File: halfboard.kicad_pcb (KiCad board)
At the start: 2 copper layers, 117.4 x 87.9 mm, 54 parts, among them U1 

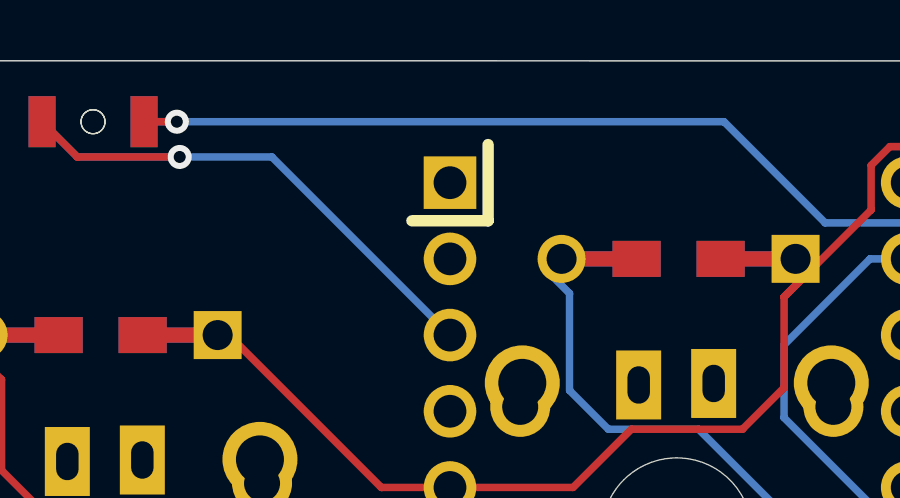
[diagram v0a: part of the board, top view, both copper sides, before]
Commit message: update gerber files
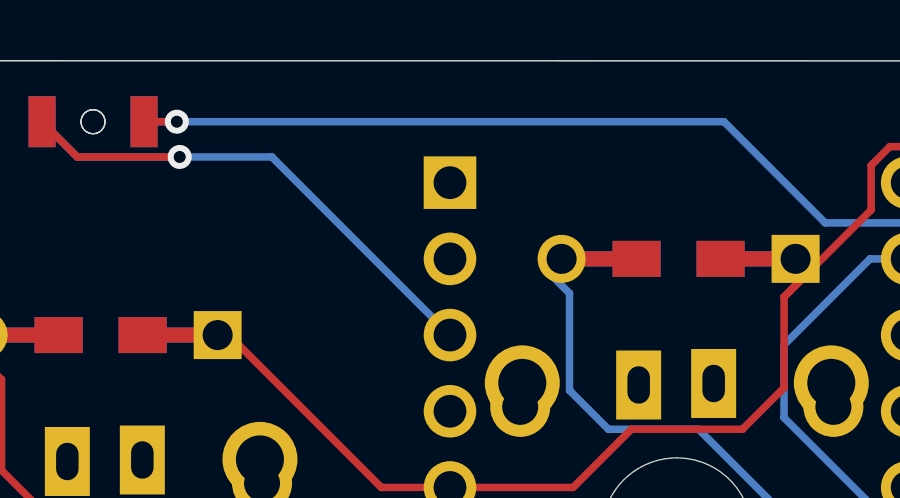
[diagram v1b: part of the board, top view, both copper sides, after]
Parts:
- removed the   at (135.4, 130.6) (x2)
- added  : , Button_Switch_SMD:SW_SPDT_PCM12, F.Cu at (135.4, 130.6)
- added  : , Button_Switch_SMD:SW_SPDT_PCM12, B.Cu at (135.4, 130.6)
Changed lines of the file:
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@@
     (add_net row3)
+  )
+  (module halfboard:ArduinoProMicro-TopSide (layer F.Cu)
+    (at 68.287231 63.5 270)
+    (fp_text reference U1 (at 0 1.625 270) (layer B.SilkS) hide
+      (effects (font (size 1.27 1.524) (thickness 0.2032)) (justify mirror))
+    )
+    (fp_text value " " (at 0 0 270) (layer F.SilkS) hide
+      (effects (font (size 1.27 1.524) (thickness 0.2032)))
+    )
+    (pad 1 thru_hole rect (at -13.97 7.62 270) (size 1.7526 1.7526) (drill 1.0922) (layers *.Cu B.SilkS))
+    (pad 2 thru_hole circle (at -11.43 7.62 270) (size 1.7526 1.7526) (drill 1.0922) (layers *.Cu *.Mask))
+    (pad 3 thru_hole circle (at -8.89 7.62 270) (size 1.7526 1.7526) (drill 1.0922) (layers *.Cu *.Mask)
+      (net 39 RESET_GND))
+    (pad 4 thru_hole circle (at -6.35 7.62 270) (size 1.7526 1.7526) (drill 1.0922) (layers *.Cu *.Mask))
+    (pad 5 thru_hole circle (at -3.81 7.62 270) (size 1.7526 1.7526) (drill 1.0922) (layers *.Cu *.Mask)
+      (net 32 row0))
+    (pad 6 thru_hole circle (at -1.27 7.62 270) (size 1.7526 1.7526) (drill 1.0922) (layers *.Cu *.Mask)
+      (net 33 row1))
+    (pad 7 thru_hole circle (at 1.27 7.62 270) (size 1.7526 1.7526) (drill 1.0922) (layers *.Cu *.Mask)
+      (net 34 row2))
+    (pad 8 thru_hole circle (at 3.81 7.62 270) (size 1.7526 1.7526) (drill 1.0922) (layers *.Cu *.Mask)
+      (net 8 row3))
+    (pad 9 thru_hole circle (at 6.35 7.62 270) (size 1.7526 1.7526) (drill 1.0922) (layers *.Cu *.Mask)
+      (net 26 col0))
+    (pad 10 thru_hole circle (at 8.89 7.62 270) (size 1.7526 1.7526) (drill 1.0922) (layers *.Cu *.Mask))
+    (pad 11 thru_hole circle (at 11.43 7.62 270) (size 1.7526 1.7526) (drill 1.0922) (layers *.Cu *.Mask)
+      (net 28 col2))
+    (pad 13 thru_hole circle (at 13.97 -7.62 270) (size 1.7526 1.7526) (drill 1.0922) (layers *.Cu *.Mask)
+      (net 30 col4))
+    (pad 14 thru_hole circle (at 11.43 -7.62 270) (size 1.7526 1.7526) (drill 1.0922) (layers *.Cu *.Mask))
+    (pad 15 thru_hole circle (at 8.89 -7.62 270) (size 1.7526 1.7526) (drill 1.0922) (layers *.Cu *.Mask)
+      (net 29 col3))
+    (pad 16 thru_hole circle (at 6.35 -7.62 270) (size 1.7526 1.7526) (drill 1.0922) (layers *.Cu *.Mask)
+      (net 31 col5))
+    (pad 17 thru_hole circle (at 3.81 -7.62 270) (size 1.7526 1.7526) (drill 1.0922) (layers *.Cu *.Mask))
+    (pad 18 thru_hole circle (at 1.27 -7.62 270) (size 1.7526 1.7526) (drill 1.0922) (layers *.Cu *.Mask))
+    (pad 19 thru_hole circle (at -1.27 -7.62 270) (size 1.7526 1.7526) (drill 1.0922) (layers *.Cu *.Mask))
+    (pad 20 thru_hole circle (at -3.81 -7.62 270) (size 1.7526 1.7526) (drill 1.0922) (layers *.Cu *.Mask))
+    (pad 21 thru_hole circle (at -6.35 -7.62 270) (size 1.7526 1.7526) (drill 1.0922) (layers *.Cu *.Mask))
+    (pad 22 thru_hole circle (at -8.89 -7.62 270) (size 1.7526 1.7526) (drill 1.0922) (layers *.Cu *.Mask)
+      (net 38 RESET))
+    (pad 23 thru_hole circle (at -11.43 -7.62 270) (size 1.7526 1.7526) (drill 1.0922) (layers *.Cu *.Mask)
+      (net 37 BAT_GND))
+    (pad 12 thru_hole circle (at 13.97 7.62 270) (size 1.7526 1.7526) (drill 1.0922) (layers *.Cu *.Mask)
+      (net 27 col1))
+    (pad 24 thru_hole circle (at -13.97 -7.62 270) (size 1.7526 1.7526) (drill 1.0922) (layers *.Cu *.Mask)
+      (net 35 BAT0))
+    (model /Users/danny/Documents/proj/custom-keyboard/kicad-libs/3d_models/Pro_Micro.wrl
+      (offset (xyz 15.23999977111816 -8.889999866485596 1.269999980926514))
+      (scale (xyz 0.395 0.395 0.395))
+      (rotate (xyz 0 0 270))
+    )
   )
   (module Button_Switch_SMD:SW_SPST_B3U-3000P-B (layer F.Cu)
@@
     (pad "" np_thru_hole circle (at 0 0 90) (size 5 5) (drill 5) (layers *.Cu *.Mask))
   )
-  (module halfboard:ArduinoProMicro-TopSide (layer F.Cu)
-    (at 68.287231 63.5 270)
-    (fp_text reference U1 (at 0 1.625 90) (layer B.SilkS) hide
-      (effects (font (size 1.27 1.524) (thickness 0.2032)) (justify mirror))
-    )
-    (fp_text value " " (at 0 0 90) (layer F.SilkS) hide
-      (effects (font (size 1.27 1.524) (thickness 0.2032)))
-    )
-    (fp_line (start -12.7 6.35) (end -12.7 8.89) (layer F.SilkS) (width 0.381))
-    (fp_line (start -15.24 6.35) (end -12.7 6.35) (layer F.SilkS) (width 0.381))
-    (pad 1 thru_hole rect (at -13.97 7.62 270) (size 1.7526 1.7526) (drill 1.0922) (layers *.Cu B.SilkS))
-    (pad 2 thru_hole circle (at -11.43 7.62 270) (size 1.7526 1.7526) (drill 1.0922) (layers *.Cu *.SilkS *.Mask))
-    (pad 3 thru_hole circle (at -8.89 7.62 270) (size 1.7526 1.7526) (drill 1.0922) (layers *.Cu *.SilkS *.Mask)
-      (net 39 RESET_GND))
-    (pad 4 thru_hole circle (at -6.35 7.62 270) (size 1.7526 1.7526) (drill 1.0922) (layers *.Cu *.SilkS *.Mask))
-    (pad 5 thru_hole circle (at -3.81 7.62 270) (size 1.7526 1.7526) (drill 1.0922) (layers *.Cu *.SilkS *.Mask)
-      (net 32 row0))
-    (pad 6 thru_hole circle (at -1.27 7.62 270) (size 1.7526 1.7526) (drill 1.0922) (layers *.Cu *.SilkS *.Mask)
-      (net 33 row1))
-    (pad 7 thru_hole circle (at 1.27 7.62 270) (size 1.7526 1.7526) (drill 1.0922) (layers *.Cu *.SilkS *.Mask)
-      (net 34 row2))
-    (pad 8 thru_hole circle (at 3.81 7.62 270) (size 1.7526 1.7526) (drill 1.0922) (layers *.Cu *.SilkS *.Mask)
-      (net 8 row3))
-    (pad 9 thru_hole circle (at 6.35 7.62 270) (size 1.7526 1.7526) (drill 1.0922) (layers *.Cu *.SilkS *.Mask)
-      (net 26 col0))
-    (pad 10 thru_hole circle (at 8.89 7.62 270) (size 1.7526 1.7526) (drill 1.0922) (layers *.Cu *.SilkS *.Mask))
-    (pad 11 thru_hole circle (at 11.43 7.62 270) (size 1.7526 1.7526) (drill 1.0922) (layers *.Cu *.SilkS *.Mask)
-      (net 28 col2))
-    (pad 13 thru_hole circle (at 13.97 -7.62 270) (size 1.7526 1.7526) (drill 1.0922) (layers *.Cu *.SilkS *.Mask)
-      (net 30 col4))
-    (pad 14 thru_hole circle (at 11.43 -7.62 270) (size 1.7526 1.7526) (drill 1.0922) (layers *.Cu *.SilkS *.Mask))
-    (pad 15 thru_hole circle (at 8.89 -7.62 270) (size 1.7526 1.7526) (drill 1.0922) (layers *.Cu *.SilkS *.Mask)
-      (net 29 col3))
-    (pad 16 thru_hole circle (at 6.35 -7.62 270) (size 1.7526 1.7526) (drill 1.0922) (layers *.Cu *.SilkS *.Mask)
-      (net 31 col5))
-    (pad 17 thru_hole circle (at 3.81 -7.62 270) (size 1.7526 1.7526) (drill 1.0922) (layers *.Cu *.SilkS *.Mask))
-    (pad 18 thru_hole circle (at 1.27 -7.62 270) (size 1.7526 1.7526) (drill 1.0922) (layers *.Cu *.SilkS *.Mask))
-    (pad 19 thru_hole circle (at -1.27 -7.62 270) (size 1.7526 1.7526) (drill 1.0922) (layers *.Cu *.SilkS *.Mask))
-    (pad 20 thru_hole circle (at -3.81 -7.62 270) (size 1.7526 1.7526) (drill 1.0922) (layers *.Cu *.SilkS *.Mask))
-    (pad 21 thru_hole circle (at -6.35 -7.62 270) (size 1.7526 1.7526) (drill 1.0922) (layers *.Cu *.SilkS *.Mask))
-    (pad 22 thru_hole circle (at -8.89 -7.62 270) (size 1.7526 1.7526) (drill 1.0922) (layers *.Cu *.SilkS *.Mask)
-      (net 38 RESET))
-    (pad 23 thru_hole circle (at -11.43 -7.62 270) (size 1.7526 1.7526) (drill 1.0922) (layers *.Cu *.SilkS *.Mask)
-      (net 37 BAT_GND))
-    (pad 12 thru_hole circle (at 13.97 7.62 270) (size 1.7526 1.7526) (drill 1.0922) (layers *.Cu *.SilkS *.Mask)
-      (net 27 col1))
-    (pad 24 thru_hole circle (at -13.97 -7.62 270) (size 1.7526 1.7526) (drill 1.0922) (layers *.Cu *.SilkS *.Mask)
-      (net 35 BAT0))
-    (model /Users/danny/Documents/proj/custom-keyboard/kicad-libs/3d_models/Pro_Micro.wrl
-      (offset (xyz 15.23999977111816 -8.889999866485596 1.269999980926514))
-      (scale (xyz 0.395 0.395 0.395))
-      (rotate (xyz 0 0 270))
-    )
-  )
   (module Button_Switch_SMD:SW_SPDT_PCM12 (layer B.Cu)
